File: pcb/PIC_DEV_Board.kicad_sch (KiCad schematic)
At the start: 8 parts, among them J1 Conn_01x08_Pin, J3 Conn_01x15_Pin, J4 Conn_01x02_Pin

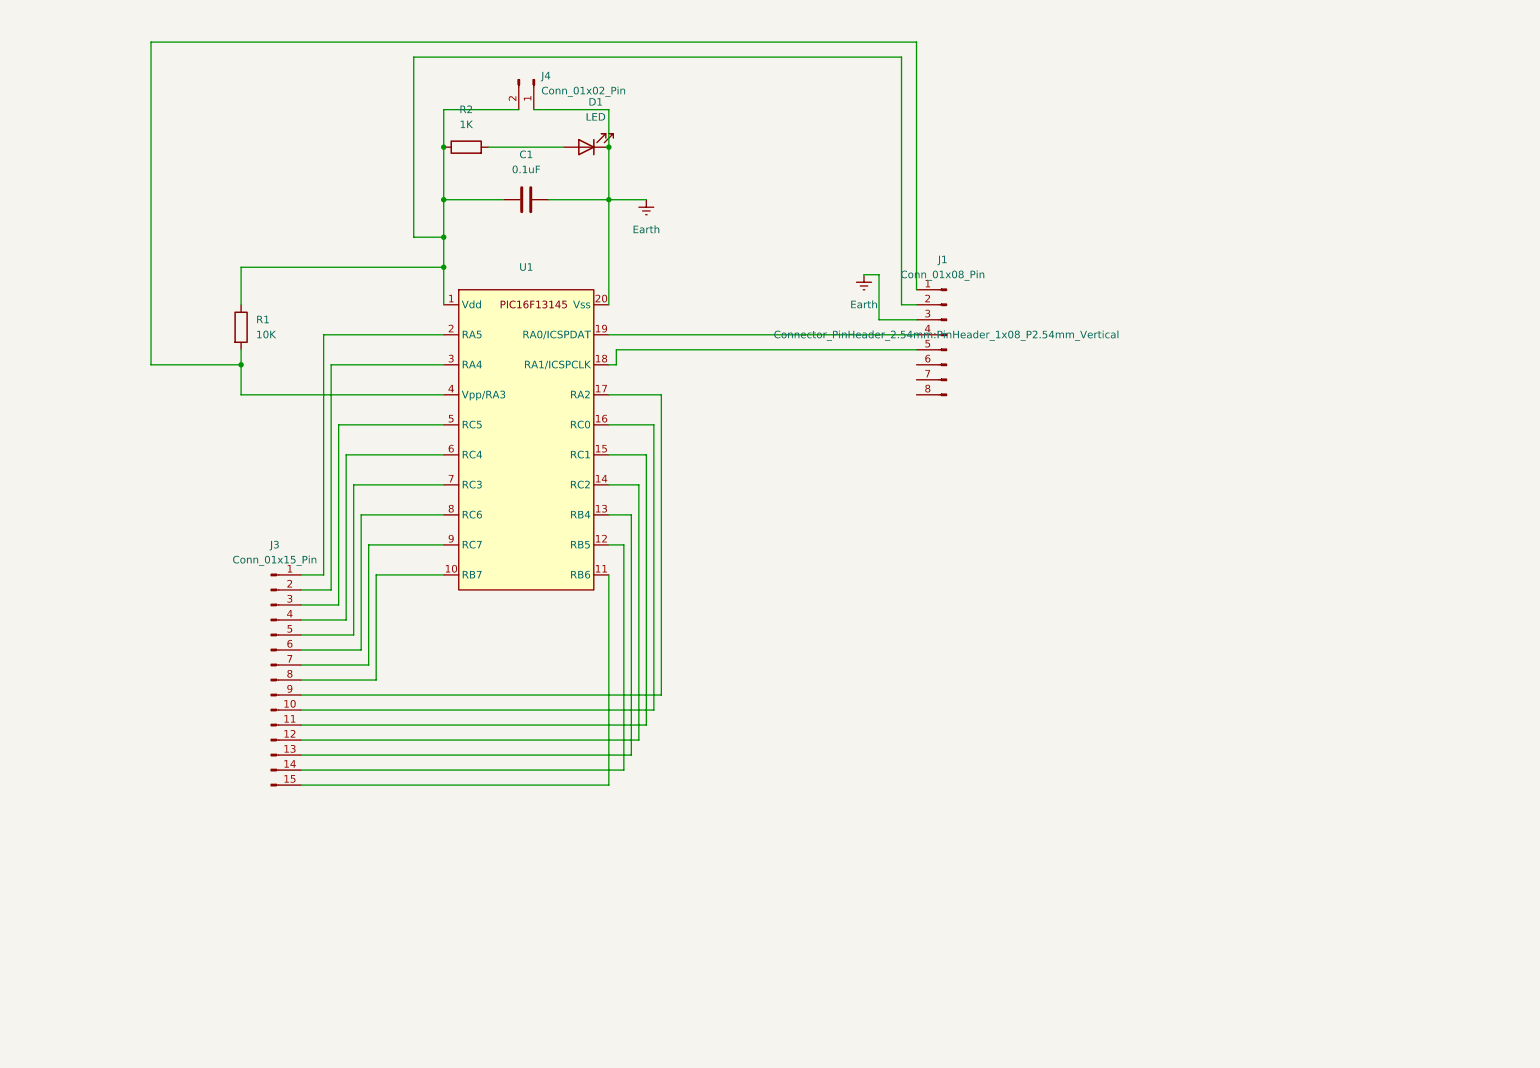
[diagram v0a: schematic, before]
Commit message: higher functionality board
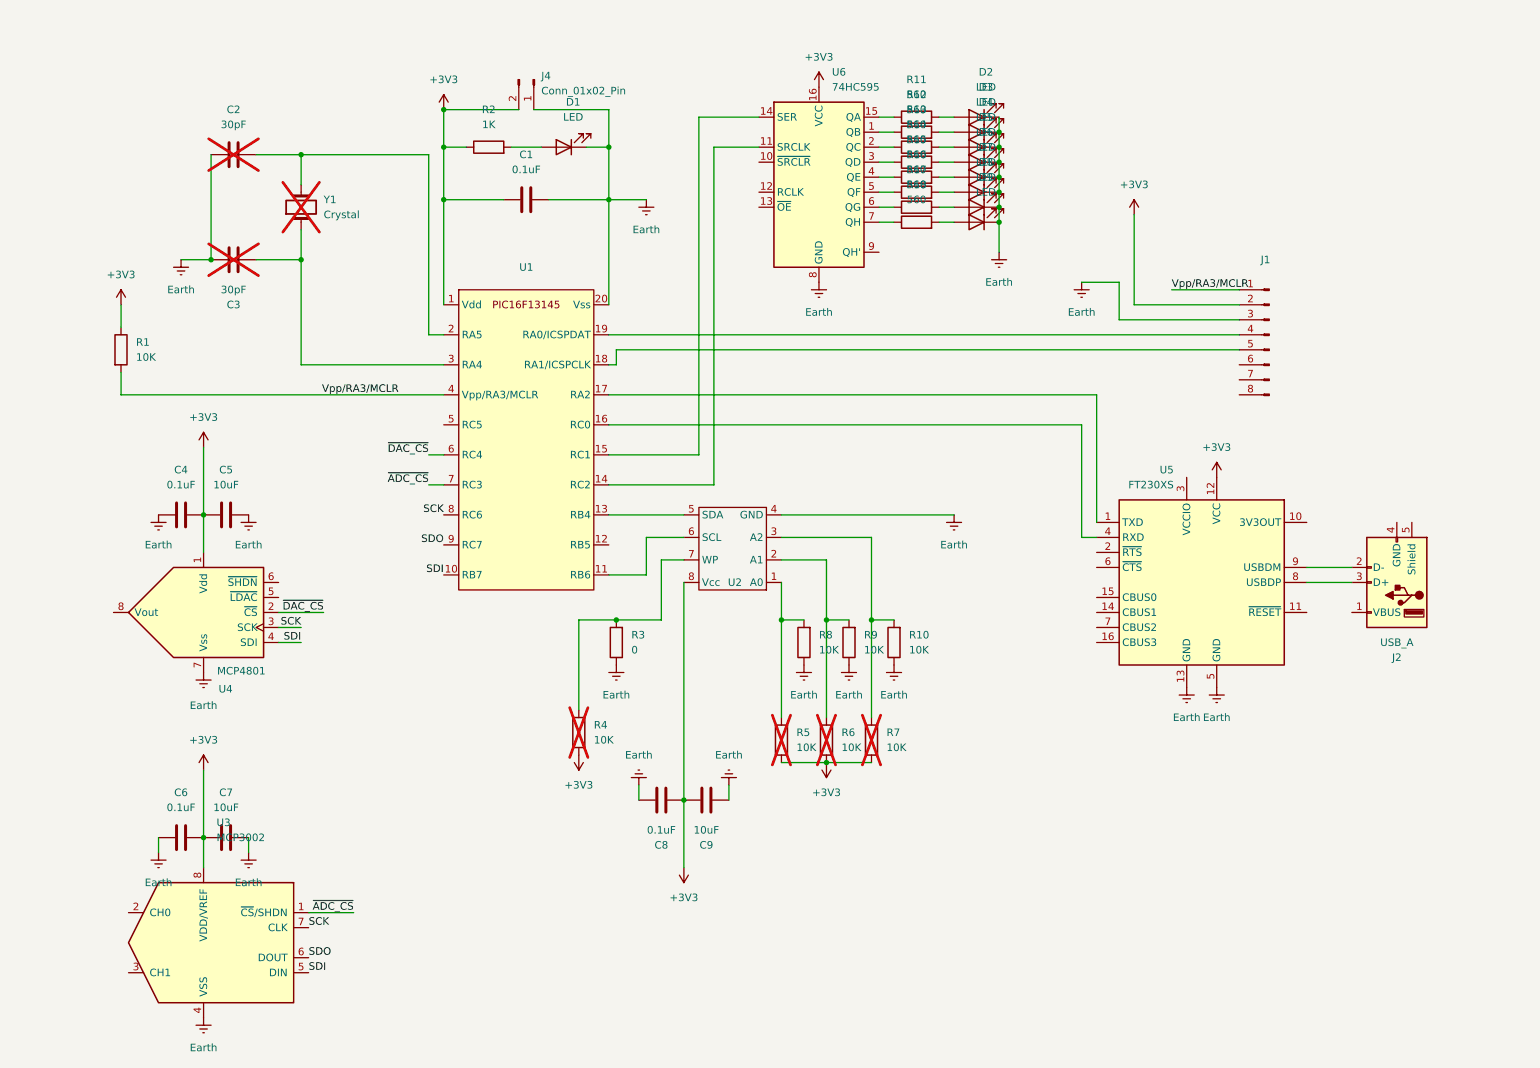
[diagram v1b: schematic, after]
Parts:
- removed J3: Conn_01x15_Pin, Connector_PinHeader_2.54mm:PinHeader_1x15_P2.54mm_Vertical, symbol Connector:Conn_01x15_Pin
- added C2, C3: 30pF, Capacitor_SMD:C_0805_2012Metric, symbol Device:C
- added C4, C6, C8: 0.1uF, Capacitor_SMD:C_0805_2012Metric, symbol Device:C
- added C5, C7, C9: 10uF, Capacitor_SMD:C_0805_2012Metric, symbol Device:C
- added D2, D3, D4, D5, D6, D7, D8, D9: LED, LED_SMD:LED_0805_2012Metric, symbol Device:LED
- added J2: USB_A, Connector_USB:USB_A_Receptacle_GCT_USB1046, symbol Connector:USB_A
- added R10, R4, R5, R6, R7, R8, R9: 10K, Resistor_SMD:R_0805_2012Metric, symbol Device:R
- added R11, R12, R13, R14, R15, R16, R17, R18: 560, Resistor_SMD:R_0805_2012Metric, symbol Device:R
- added R3: 0, Resistor_SMD:R_0805_2012Metric, symbol Device:R
- added U2: ~, Package_SO:SOIC-8_3.9x4.9mm_P1.27mm, symbol myCustomParts:AT24C01D
- added U3: MCP3002, Package_SO:SOIC-8_3.9x4.9mm_P1.27mm, symbol Analog_ADC:MCP3002
- added U4: MCP4801, Package_SO:SOIC-8_3.9x4.9mm_P1.27mm, symbol Analog_DAC:MCP4801
- added U5: FT230XS, Package_SO:SSOP-16_3.9x4.9mm_P0.635mm, symbol Interface_USB:FT230XS
- added U6: 74HC595, Package_SO:SOIC-16_3.9x9.9mm_P1.27mm, symbol 74xx:74HC595
- added Y1: Crystal, symbol Device:Crystal
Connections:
- net Earth: now also C2.1, C3.1, C4.2, C5.1, C6.2, C7.1, C8.2, C9.1, D2.1 (K), D3.1 (K), D4.1 (K), D5.1 (K), D6.1 (K), D7.1 (K), D8.1 (K), D9.1 (K), R10.1, R3.1, R8.1, R9.1, U2.4 (GND), U3.4 (VSS), U4.7 (Vss), U5.13 (GND), U5.5 (GND), U6.8 (GND)
- net +3V3: now reaches C1.2, J1.2 (Pin_2), J4.2 (Pin_2), R1.1, R2.1, U1.1 (Vdd)
- net +3V3: now also C4.1, C5.2, C6.1, C7.2, C8.1, C9.2, R4.1, R5.1, R6.1, R7.1, U2.8 (Vcc), U3.8 (VDD/VREF), U4.1 (Vdd), U5.12 (VCC), U6.16 (VCC)
- net Vpp/RA3/MCLR: now reaches R1.2, U1.4 (Vpp/RA3/MCLR)
- net Vpp/RA3/MCLR: no longer J1.1 (Pin_1)
- net at U1.2 (RA5): now also C2.2, Y1.2
- net at U1.16 (RC0): now also U5.4 (RXD)
- net at U1.15 (RC1): now also U6.14 (SER)
- net at U1.14 (RC2): now also U6.11 (SRCLK)
- net at U1.13 (RB4): now also U2.5 (SDA)
- net at U1.11 (RB6): now also U2.6 (SCL)
- net at U1.3 (RA4): now also C3.2, Y1.1
- net ~{DAC_CS}: now reaches U1.6 (RC4)
- net ~{DAC_CS}: now also U4.2 (~{CS})
- net ~{ADC_CS}: now reaches U1.7 (RC3)
- net ~{ADC_CS}: now also U3.1 (~{CS}/SHDN)
- net SCK: now reaches U1.8 (RC6)
- net SCK: now also U3.7 (CLK), U4.3 (SCK)
- net SDO: now reaches U1.9 (RC7)
- net SDO: now also U3.6 (DOUT)
- net SDI: now reaches U1.10 (RB7)
- net SDI: now also U3.5 (DIN), U4.4 (SDI)
- net at U1.17 (RA2): now also U5.1 (TXD)
- new net: D5.2 (A), R14.2
- new net: R6.2, R9.2, U2.2 (A1)
- new net: J2.3 (D+), U5.8 (USBDP)
- new net: J2.2 (D-), U5.9 (USBDM)
- new net: R14.1, U6.3 (QD)
- new net: R15.1, U6.4 (QE)
- new net: D6.2 (A), R15.2
- new net: R3.2, R4.2, U2.7 (WP)
- new net: D2.2 (A), R11.2
- new net: D4.2 (A), R13.2
- new net: R10.2, R7.2, U2.3 (A2)
- new net: D7.2 (A), R16.2
- new net: R16.1, U6.5 (QF)
- new net: D8.2 (A), R17.2
- new net: R5.2, R8.2, U2.1 (A0)
- new net: R13.1, U6.2 (QC)
- new net: R17.1, U6.6 (QG)
- new net: R11.1, U6.15 (QA)
- new net: R12.1, U6.1 (QB)
- new net: R18.1, U6.7 (QH)
- new net: D9.2 (A), R18.2
- new net: D3.2 (A), R12.2
- new net Vpp/RA3/MCLR: J1.1 (Pin_1)
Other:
- moved on the sheet: D1, J1, R1, R2

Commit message: size reduction
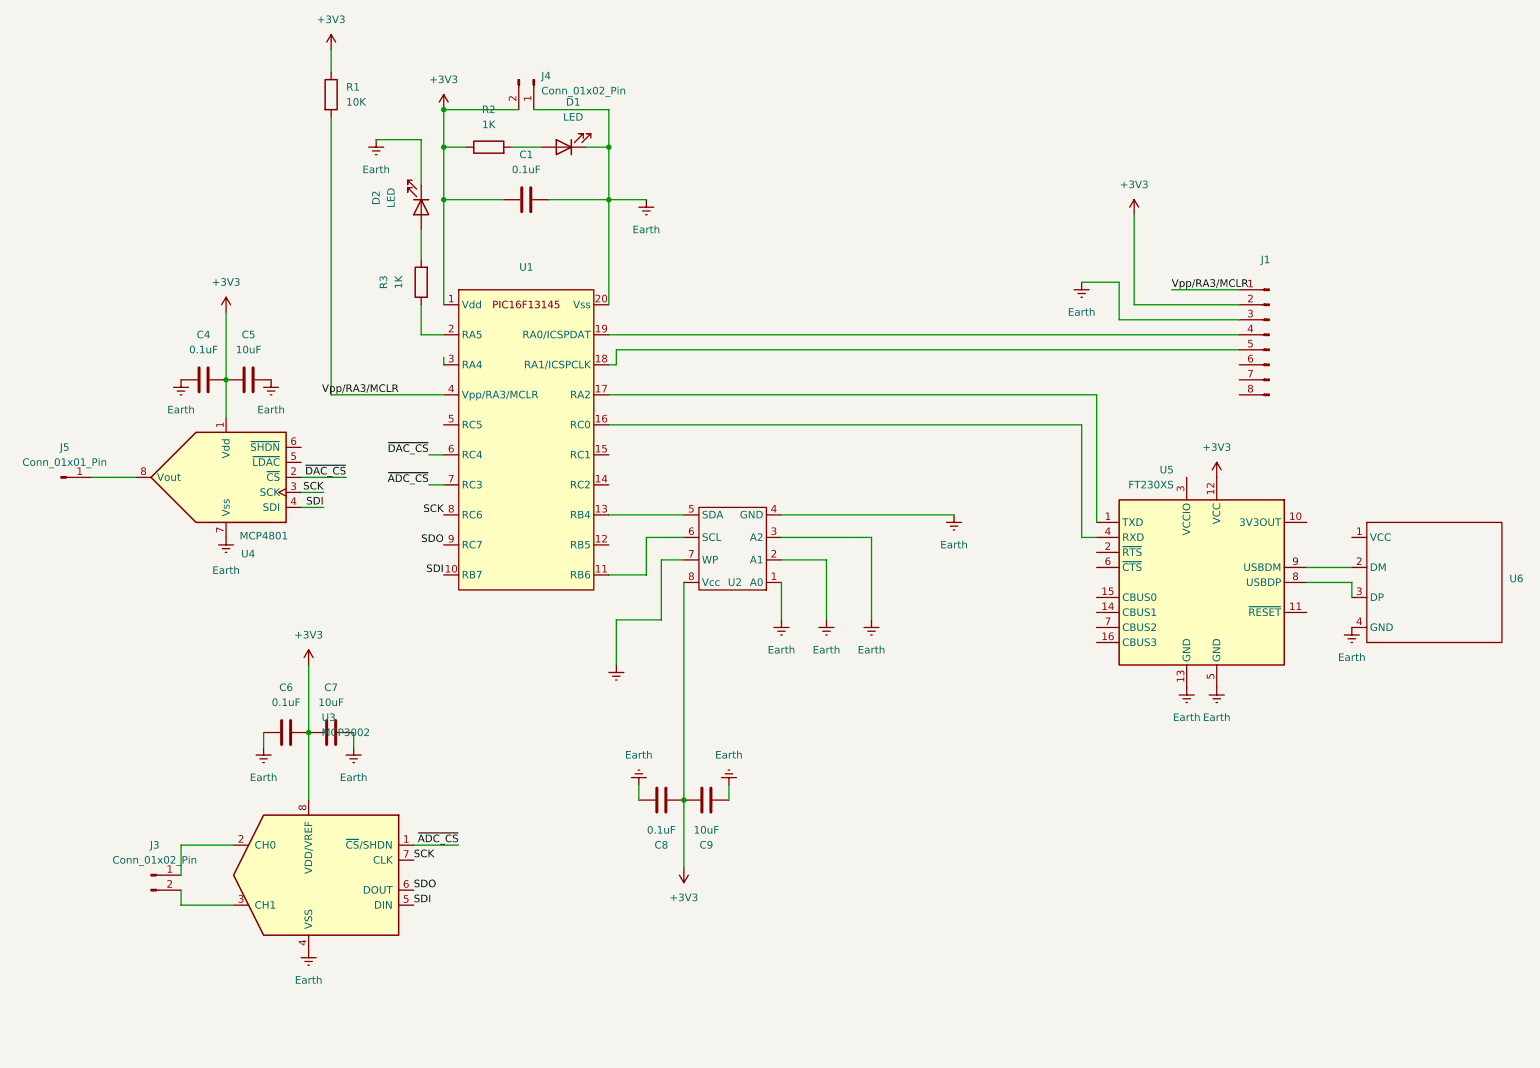
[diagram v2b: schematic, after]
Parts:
- removed C2, C3: 30pF, Capacitor_SMD:C_0805_2012Metric, symbol Device:C
- removed D3, D4, D5, D6, D7, D8, D9: LED, LED_SMD:LED_0805_2012Metric, symbol Device:LED
- removed J2: USB_A, Connector_USB:USB_A_Receptacle_GCT_USB1046, symbol Connector:USB_A
- removed R10, R4, R5, R6, R7, R8, R9: 10K, Resistor_SMD:R_0805_2012Metric, symbol Device:R
- removed R11, R12, R13, R14, R15, R16, R17, R18: 560, Resistor_SMD:R_0805_2012Metric, symbol Device:R
- removed U6: 74HC595, Package_SO:SOIC-16_3.9x9.9mm_P1.27mm, symbol 74xx:74HC595
- removed Y1: Crystal, symbol Device:Crystal
- added J3: Conn_01x02_Pin, Connector_PinHeader_2.54mm:PinHeader_1x02_P2.54mm_Vertical, symbol Connector:Conn_01x02_Pin
- added J5: Conn_01x01_Pin, Connector_PinHeader_2.54mm:PinHeader_1x01_P2.54mm_Vertical, symbol Connector:Conn_01x01_Pin
- added U6: ~, myCustomFootprints:USB-A1HSB6, symbol myCustomParts:USB-A1HSB6
- R3: value 0 -> 1K
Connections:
- net Earth: now also U2.1 (A0), U2.2 (A1), U2.3 (A2), U2.7 (WP), U6.4 (GND); no longer R3.1
- net at U5.8 (USBDP): now also U6.3 (DP)
- net at U5.9 (USBDM): now also U6.2 (DM)
- net at R3.2: now also D2.2 (A); no longer U2.7 (WP)
- net at U4.8 (Vout): now also J5.1 (Pin_1)
- net at U1.2 (RA5): now also R3.1
- net at U3.2 (CH0): now also J3.1 (Pin_1)
- net at U3.3 (CH1): now also J3.2 (Pin_2)
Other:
- moved on the sheet: C4, C5, C6, C7, R1, U3, U4
